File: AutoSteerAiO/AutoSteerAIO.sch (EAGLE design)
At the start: 87 parts, among them K4 CB1A-P-12V, U1 VX7805-1000

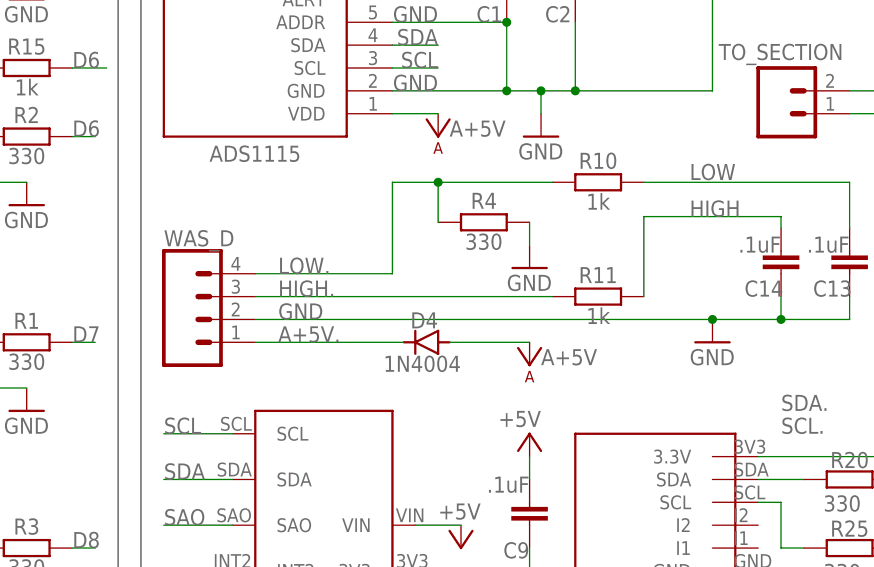
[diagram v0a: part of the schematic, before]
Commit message: Add files via upload
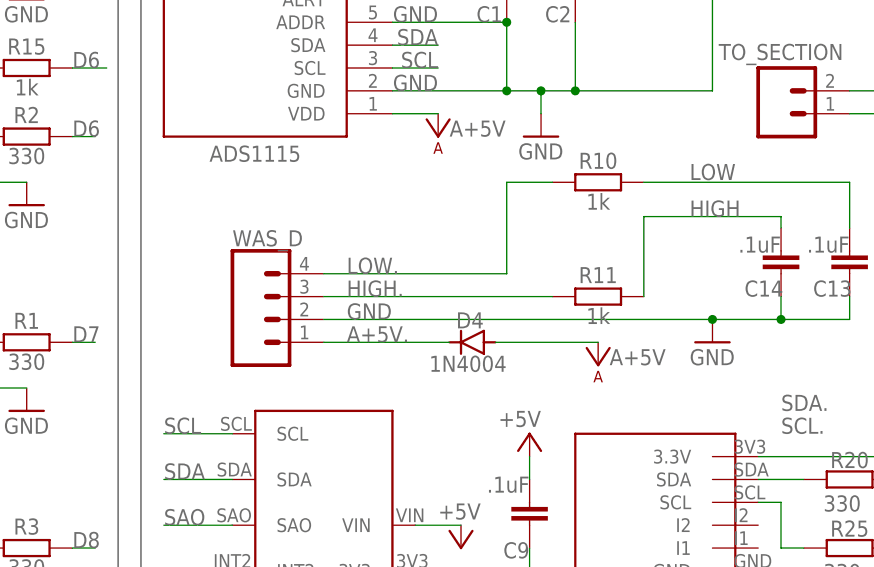
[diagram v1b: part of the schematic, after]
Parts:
- removed R4: 330, resistor:R-EU_0207/7
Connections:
- net GND: no longer R4.2
- net LOW.: no longer R4.1
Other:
- moved on the sheet: D4, WAS_D
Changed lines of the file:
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@@
 <?xml version="1.0" encoding="utf-8"?>
 <!DOCTYPE eagle SYSTEM "eagle.dtd">
-<eagle version="9.5.2">
+<eagle version="9.6.1">
 <drawing>
 <settings>
@@
 <attribute name="OC_NEWARK" value="unknown"/>
 </part>
-<part name="R4" library="resistor" library_urn="urn:adsk.eagle:library:348" deviceset="R-EU_" device="0207/7" package3d_urn="urn:adsk.eagle:package:23493/2" value="330">
-<attribute name="MF" value=""/>
-<attribute name="MPN" value=""/>
-<attribute name="OC_NEWARK" value="unknown"/>
-</part>
 <part name="TO_SECTION" library="SparkFun-Connectors" library_urn="urn:adsk.eagle:library:513" deviceset="CONN_02" device="" package3d_urn="urn:adsk.eagle:package:38039/1" value="CONNECTOR 1x2 PINS">
 <attribute name="MF" value=""/>
@@
 <part name="GND26" library="supply1" library_urn="urn:adsk.eagle:library:371" deviceset="GND" device=""/>
 <part name="P+14" library="supply1" library_urn="urn:adsk.eagle:library:371" deviceset="+5V" device=""/>
-<part name="GND27" library="supply1" library_urn="urn:adsk.eagle:library:371" deviceset="GND" device=""/>
 <part name="GND29" library="supply1" library_urn="urn:adsk.eagle:library:371" deviceset="GND" device=""/>
 <part name="GND28" library="supply1" library_urn="urn:adsk.eagle:library:371" deviceset="GND" device=""/>
@@
 <attribute name="MPN" x="71.12" y="177.8" size="1.778" layer="96" display="off"/>
 </instance>
-<instance part="WAS_D" gate="G$1" x="66.04" y="142.24" smashed="yes">
-<attribute name="NAME" x="60.96" y="150.368" size="1.778" layer="95" font="vector"/>
-<attribute name="OC_NEWARK" x="66.04" y="142.24" size="1.778" layer="96" display="off"/>
-<attribute name="MF" x="66.04" y="142.24" size="1.778" layer="96" display="off"/>
-<attribute name="MPN" x="66.04" y="142.24" size="1.778" layer="96" display="off"/>
+<instance part="WAS_D" gate="G$1" x="73.66" y="142.24" smashed="yes">
+<attribute name="NAME" x="68.58" y="150.368" size="1.778" layer="95" font="vector"/>
+<attribute name="OC_NEWARK" x="73.66" y="142.24" size="1.778" layer="96" display="off"/>
+<attribute name="MF" x="73.66" y="142.24" size="1.778" layer="96" display="off"/>
+<attribute name="MPN" x="73.66" y="142.24" size="1.778" layer="96" display="off"/>
 </instance>
 <instance part="STEER-SWITCH" gate="J$1" x="-5.08" y="157.48" smashed="yes">
@@
 <attribute name="MPN" x="129.54" y="147.32" size="1.778" layer="96" display="off"/>
 </instance>
-<instance part="D4" gate="1" x="90.17" y="139.7" smashed="yes" rot="R180">
-<attribute name="NAME" x="91.44" y="143.0274" size="1.778" layer="95" rot="R180"/>
-<attribute name="VALUE" x="93.98" y="138.2014" size="1.778" layer="96" rot="R180"/>
-<attribute name="OC_NEWARK" x="90.17" y="139.7" size="1.778" layer="96" display="off"/>
-<attribute name="MF" x="90.17" y="139.7" size="1.778" layer="96" display="off"/>
-<attribute name="MPN" x="90.17" y="139.7" size="1.778" layer="96" display="off"/>
+<instance part="D4" gate="1" x="95.25" y="139.7" smashed="yes" rot="R180">
+<attribute name="NAME" x="96.52" y="143.0274" size="1.778" layer="95" rot="R180"/>
+<attribute name="VALUE" x="99.06" y="138.2014" size="1.778" layer="96" rot="R180"/>
+<attribute name="OC_NEWARK" x="95.25" y="139.7" size="1.778" layer="96" display="off"/>
+<attribute name="MF" x="95.25" y="139.7" size="1.778" layer="96" display="off"/>
+<attribute name="MPN" x="95.25" y="139.7" size="1.778" layer="96" display="off"/>
 </instance>
 <instance part="P+10" gate="1" x="7.62" y="167.64" smashed="yes">
@@
 <attribute name="MPN" x="27.94" y="220.98" size="1.778" layer="96" display="off"/>
 </instance>
-<instance part="R4" gate="G$1" x="96.52" y="153.035" smashed="yes">
-<attribute name="NAME" x="96.52" y="154.5336" size="1.778" layer="95" rot="R180" align="top-center"/>
-<attribute name="VALUE" x="96.52" y="151.765" size="1.778" layer="95" rot="R180" align="bottom-center"/>
-<attribute name="OC_NEWARK" x="96.52" y="153.035" size="1.778" layer="96" display="off"/>
-<attribute name="MF" x="96.52" y="153.035" size="1.778" layer="96" display="off"/>
-<attribute name="MPN" x="96.52" y="153.035" size="1.778" layer="96" display="off"/>
-</instance>
 <instance part="TO_SECTION" gate="G$1" x="129.54" y="165.1" smashed="yes">
 <attribute name="NAME" x="129.54" y="171.958" size="1.778" layer="95" font="vector" align="center"/>
@@
 </instance>
 <instance part="P+14" gate="1" x="190.5" y="179.07" smashed="yes" rot="R180"/>
-<instance part="GND27" gate="1" x="101.6" y="147.955" smashed="yes">
-<attribute name="VALUE" x="99.06" y="145.415" size="1.778" layer="96"/>
-</instance>
 <instance part="GND29" gate="1" x="121.92" y="139.7" smashed="yes">
 <attribute name="VALUE" x="119.38" y="137.16" size="1.778" layer="96"/>
@@
 <attribute name="VALUE" x="115.57" y="238.76" size="1.778" layer="96" rot="R270"/>
 </instance>
-<instance part="U$15" gate="G$1" x="101.6" y="137.16" smashed="yes" rot="R180">
-<attribute name="VALUE" x="102.87" y="137.16" size="1.778" layer="96"/>
+<instance part="U$15" gate="G$1" x="109.22" y="137.16" smashed="yes" rot="R180">
+<attribute name="VALUE" x="110.49" y="137.16" size="1.778" layer="96"/>
 </instance>
 <instance part="U$16" gate="G$1" x="91.44" y="162.56" smashed="yes" rot="R180">
@@
 <segment>
 <pinref part="WAS_D" gate="G$1" pin="3"/>
-<label x="73.66" y="144.78" size="1.778" layer="95"/>
+<label x="81.28" y="144.78" size="1.778" layer="95"/>
 <pinref part="R11" gate="G$1" pin="1"/>
-<wire x1="71.12" y1="144.78" x2="104.14" y2="144.78" width="0.1524" layer="91"/>
+<wire x1="78.74" y1="144.78" x2="104.14" y2="144.78" width="0.1524" layer="91"/>
 </segment>
 </net>
@@
 <segment>
 <pinref part="WAS_D" gate="G$1" pin="4"/>
-<label x="73.66" y="147.32" size="1.778" layer="95"/>
+<label x="81.28" y="147.32" size="1.778" layer="95"/>
 <pinref part="R10" gate="G$1" pin="1"/>
-<wire x1="71.12" y1="147.32" x2="86.36" y2="147.32" width="0.1524" layer="91"/>
-<wire x1="104.14" y1="157.48" x2="91.44" y2="157.48" width="0.1524" layer="91"/>
-<wire x1="91.44" y1="157.48" x2="86.36" y2="157.48" width="0.1524" layer="91"/>
-<wire x1="86.36" y1="157.48" x2="86.36" y2="147.32" width="0.1524" layer="91"/>
-<pinref part="R4" gate="G$1" pin="1"/>
-<wire x1="91.44" y1="153.035" x2="91.44" y2="157.48" width="0.1524" layer="91"/>
-<junction x="91.44" y="157.48"/>
+<wire x1="78.74" y1="147.32" x2="99.06" y2="147.32" width="0.1524" layer="91"/>
+<wire x1="104.14" y1="157.48" x2="99.06" y2="157.48" width="0.1524" layer="91"/>
+<wire x1="99.06" y1="157.48" x2="99.06" y2="147.32" width="0.1524" layer="91"/>
 </segment>
 </net>
@@
 <segment>
 <pinref part="WAS_D" gate="G$1" pin="2"/>
-<label x="73.66" y="142.24" size="1.778" layer="95"/>
+<label x="81.28" y="142.24" size="1.778" layer="95"/>
 <pinref part="C13" gate="G$1" pin="1"/>
 <pinref part="C14" gate="G$1" pin="1"/>
@@
 <junction x="129.54" y="142.24"/>
 <wire x1="129.54" y1="142.24" x2="137.16" y2="142.24" width="0.1524" layer="91"/>
-<wire x1="71.12" y1="142.24" x2="121.92" y2="142.24" width="0.1524" layer="91"/>
+<wire x1="78.74" y1="142.24" x2="121.92" y2="142.24" width="0.1524" layer="91"/>
 <pinref part="GND29" gate="1" pin="GND"/>
 <junction x="121.92" y="142.24"/>
@@
 </segment>
 <segment>
-<pinref part="R4" gate="G$1" pin="2"/>
-<pinref part="GND27" gate="1" pin="GND"/>
-<wire x1="101.6" y1="153.035" x2="101.6" y2="150.495" width="0.1524" layer="91"/>
-</segment>
-<segment>
 <pinref part="STEER-SWITCH" gate="J$1" pin="1"/>
 <pinref part="GND16" gate="1" pin="GND"/>
@@
 <segment>
 <pinref part="WAS_D" gate="G$1" pin="1"/>
-<wire x1="71.12" y1="139.7" x2="87.63" y2="139.7" width="0.1524" layer="91"/>
+<wire x1="78.74" y1="139.7" x2="92.71" y2="139.7" width="0.1524" layer="91"/>
 <pinref part="D4" gate="1" pin="C"/>
-<label x="73.66" y="139.7" size="1.778" layer="95"/>
+<label x="81.28" y="139.7" size="1.778" layer="95"/>
 </segment>
 </net>
@@
 <segment>
 <pinref part="D4" gate="1" pin="A"/>
-<wire x1="92.71" y1="139.7" x2="101.6" y2="139.7" width="0.1524" layer="91"/>
+<wire x1="97.79" y1="139.7" x2="109.22" y2="139.7" width="0.1524" layer="91"/>
 <pinref part="U$15" gate="G$1" pin="A+5V"/>
 </segment>

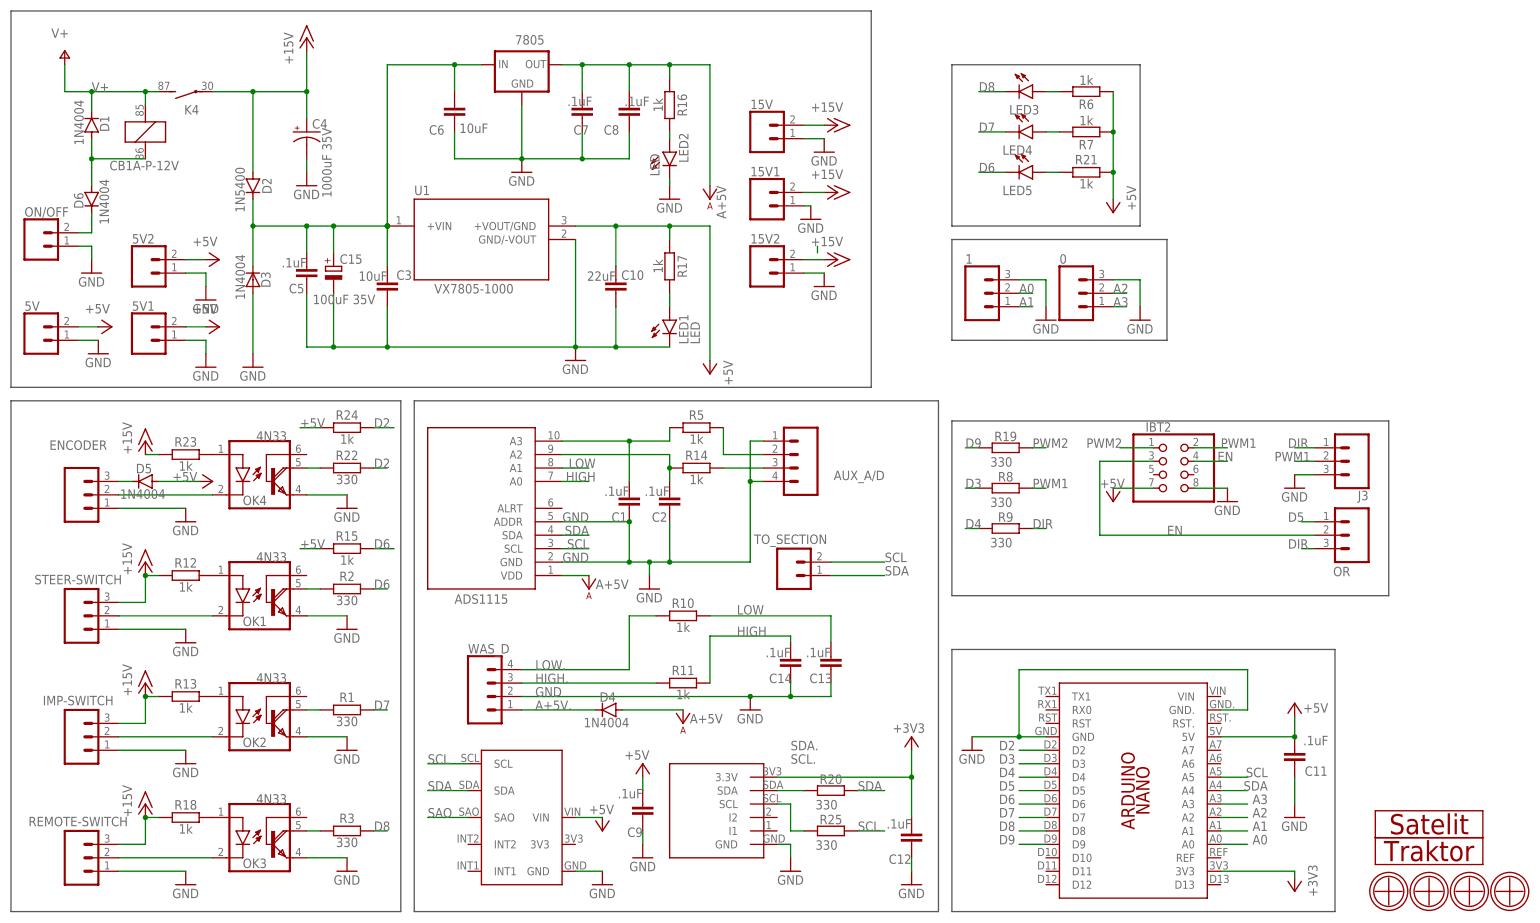
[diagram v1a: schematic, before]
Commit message: Add files via upload
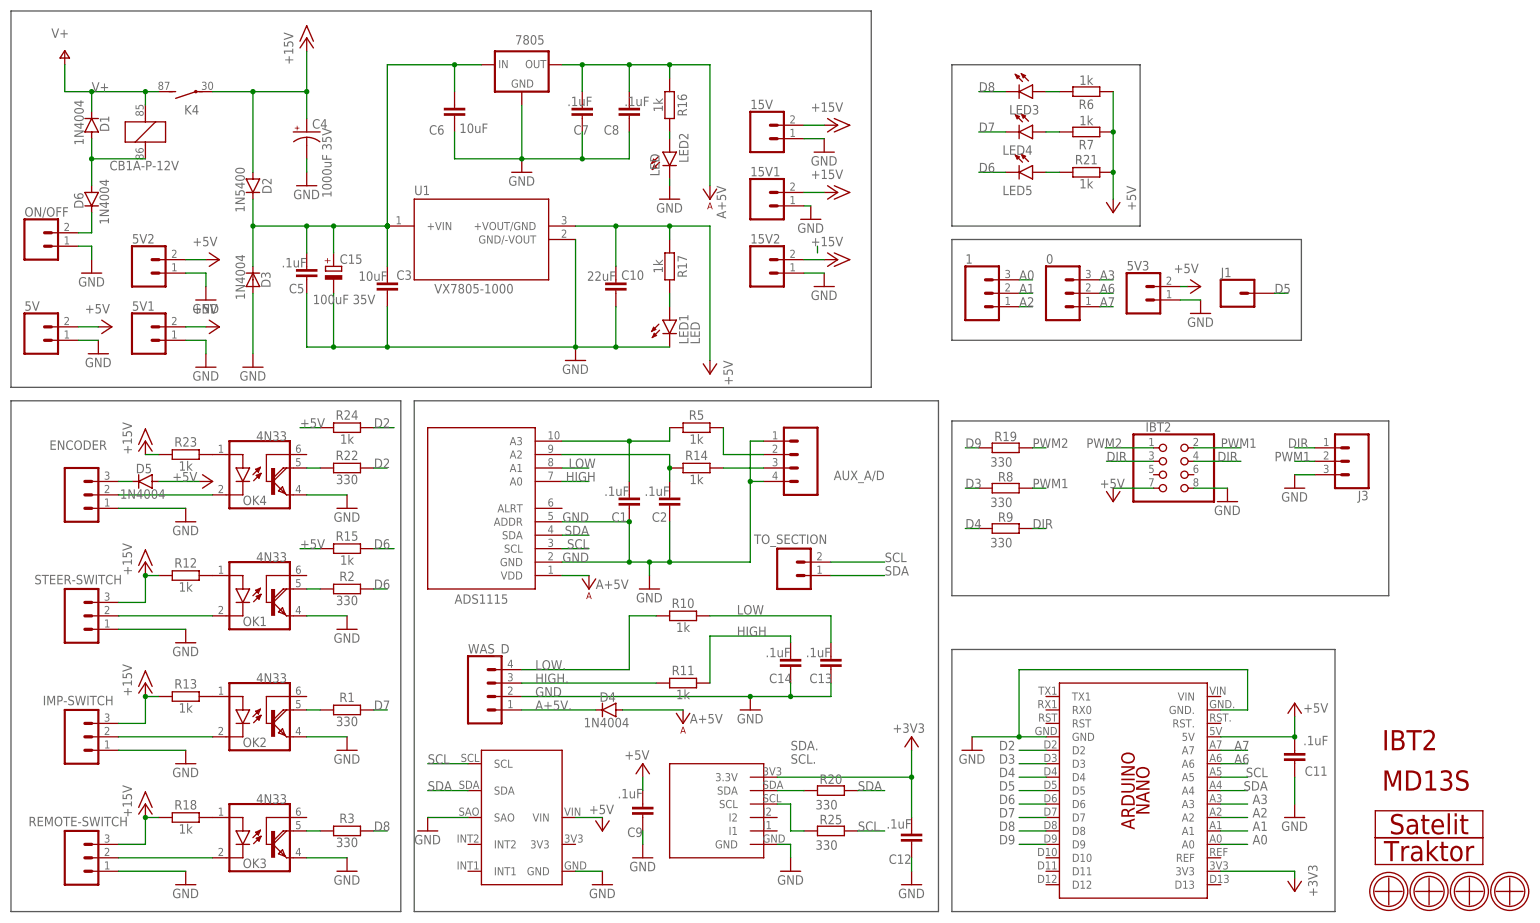
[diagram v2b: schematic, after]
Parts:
- removed OR: CONNECTOR 1x3 PINS, SparkFun-Connectors:CONN_03
- added 5V3: CONNECTOR 1x2 PINS, SparkFun-Connectors:CONN_02
- added J1: (no value), SparkFun-Connectors:CONN_01
- added U$1: MD13S, #Motor Drivers:MD13S
- added U$2: IBT2, #Motor Drivers:IBT2
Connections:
- removed net EN: IBT2.3, IBT2.4, OR.2
- removed net SAO: MMA8542.SAO
- new net A6: 0.2, PCB1.A6
- new net A7: 0.1, PCB1.A7
- net +5V: now also 5V3.2
- net A0: now also 1.3; no longer 1.2
- net A1: now also 1.2; no longer 1.1
- net A2: now also 1.1; no longer 0.2
- net A3: now also 0.3; no longer 0.1
- net D5: now also J1.1; no longer OR.1
- net DIR: now also IBT2.3, IBT2.4; no longer OR.3
- net GND: now also 5V3.1, MMA8542.SAO; no longer 0.3, 1.3
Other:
- moved on the sheet: 0
